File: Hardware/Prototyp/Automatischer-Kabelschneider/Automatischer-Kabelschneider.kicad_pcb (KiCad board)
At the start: 4 copper layers, 4 parts, among them J1 USB_C_Receptacle_USB2.0_16P, U1 AP63203WU, U2 ESP32-S3-WROOM-2

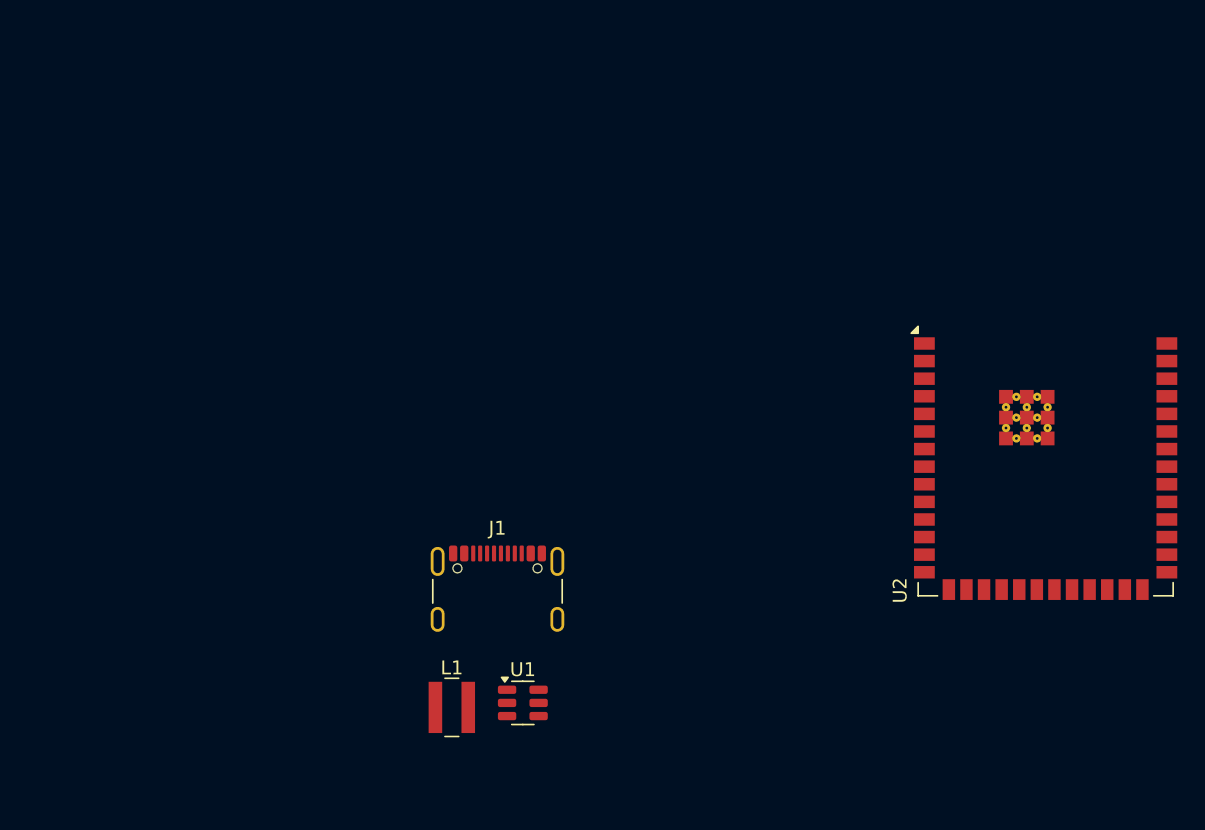
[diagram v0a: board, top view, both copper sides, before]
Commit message: 20240410
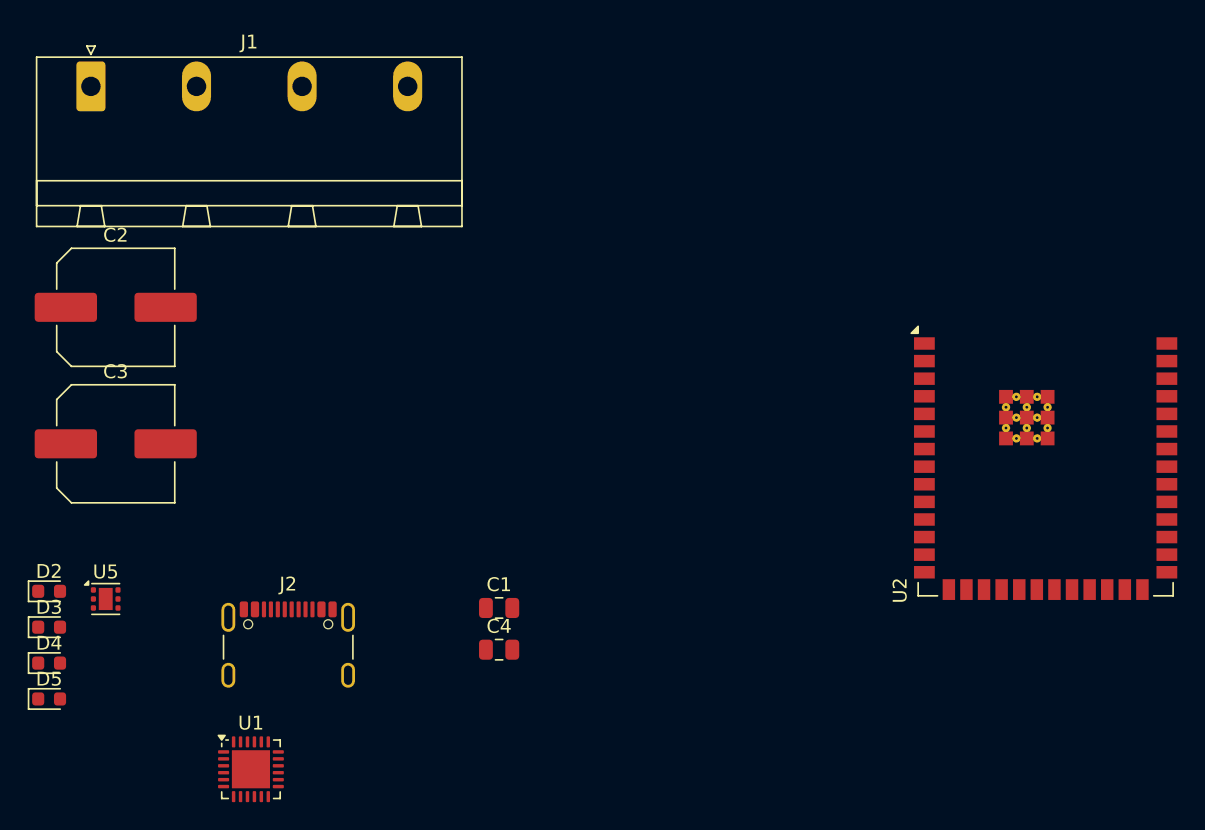
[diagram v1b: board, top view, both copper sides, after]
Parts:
- removed L1: 3u9, Inductor_SMD:L_Wuerth_MAPI-4020
- added C1: 100n, Capacitor_SMD:C_0805_2012Metric, F.Cu at (63.9, 71.7)
- added C2: 470u, Capacitor_SMD:C_Elec_8x10.2, F.Cu at (36.3, 50.0)
- added C3: 470u, Capacitor_SMD:C_Elec_8x10.2, F.Cu at (36.3, 59.8)
- added C4: 1u, Capacitor_SMD:C_0805_2012Metric, F.Cu at (63.9, 74.7)
- added D2: D_TVS, Diode_SMD:D_0603_1608Metric, F.Cu at (31.5, 70.5)
- added D3: D_TVS, Diode_SMD:D_0603_1608Metric, F.Cu at (31.5, 73.1)
- added D4: D_TVS, Diode_SMD:D_0603_1608Metric, F.Cu at (31.5, 75.6)
- added D5: D_TVS, Diode_SMD:D_0603_1608Metric, F.Cu at (31.5, 78.2)
- added J2: USB_C_Receptacle_USB2.0_16P, Connector_USB:USB_C_Receptacle_GCT_USB4105-xx-A_16P_TopMnt_Horizontal, F.Cu at (48.7, 75.4)
- added U5: TVS2200DRV, Package_SON:WSON-6-1EP_2x2mm_P0.65mm_EP1x1.6mm, F.Cu at (35.6, 71.0)
- J1: value USB_C_Receptacle_USB2.0_16P -> Conn_01x04; footprint Connector_USB:USB_C_Receptacle_GCT_USB4105-xx-A_16P_TopMnt_Horizontal -> Connector_Phoenix_GMSTB:PhoenixContact_GMSTBA_2,5_4-G-7,62_1x04_P7.62mm_Horizontal
- U1: value AP63203WU -> CYPD3177-24LQ; footprint Package_TO_SOT_SMD:TSOT-23-6 -> Package_DFN_QFN:QFN-24-1EP_4x4mm_P0.5mm_EP2.75x2.75mm
- moved J1 47.5 mm to (34.5, 34.0)
- moved U1 20.2 mm to (46.0, 83.3)
